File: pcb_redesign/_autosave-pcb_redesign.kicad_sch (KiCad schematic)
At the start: 6 parts, among them U1 ESP32-S3-WROOM-1

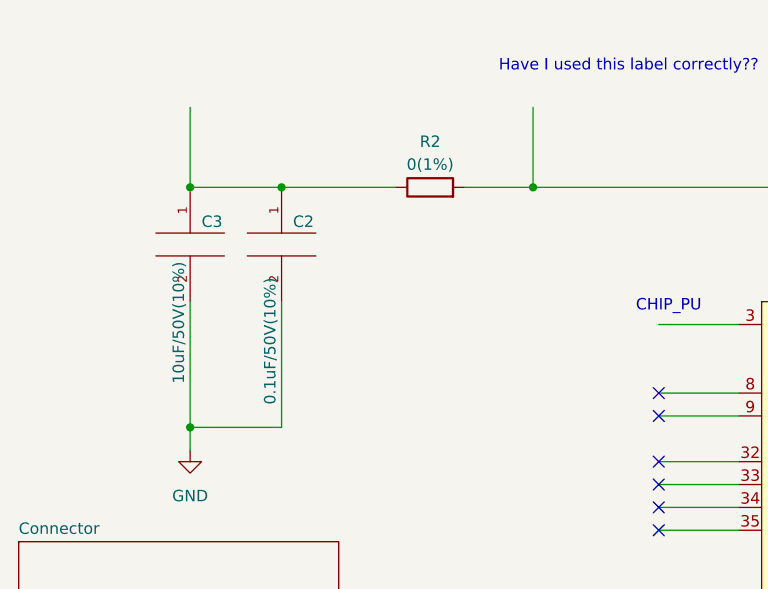
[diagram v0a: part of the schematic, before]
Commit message: 5.55pm 11.05
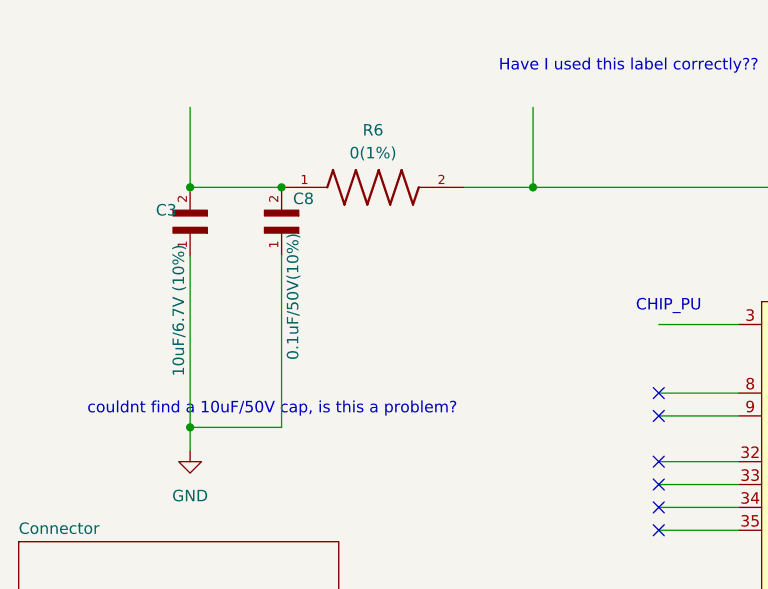
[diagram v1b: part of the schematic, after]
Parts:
- removed C2: 0.1uF/50V(10%), symbol pspice:C
- removed C3: 10uF/50V(10%), 10uF_cap_0805:CAPC2012X140N, symbol pspice:C
- removed R2: 0(1%), symbol Device:R
- added C3: 10uF/6.7V (10%), CAPC1608X90N, symbol 10uf_cap_0603:CL10A106MQ8NNNC
- added C8: 0.1uF/50V(10%), 1uF_cap_0603:CL10A105KB8NNNC, symbol 0.1uF_cap_0603:CL10B104KB8NNNL
- added R6: 0(1%), RESC1508X55N, symbol 0_ohm_0603:RMCF0603ZT0R00
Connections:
- net GND: now also C3.1, C8.1
- net at U1.2 (3V3): now also R6.2
- new net: C3.2, C8.2, R6.1
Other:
- note added: "couldnt find a 10uF/50V cap, is this a problem?"
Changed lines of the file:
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@@
 (kicad_sch (version 20230121) (generator eeschema)
   (paper "A4")
+  (junction (at 46.99 43.18) (diameter 0) (color 0 0 0 0)
+  )
   (junction (at 36.83 43.18) (diameter 0) (color 0 0 0 0)
   )
   (junction (at 36.83 69.85) (diameter 0) (color 0 0 0 0)
-  )
-  (junction (at 46.99 43.18) (diameter 0) (color 0 0 0 0)
   )
   (junction (at 66.04 175.26) (diameter 0) (color 0 0 0 0)
@@
     (stroke (width 0) (type default))
   )
+  (wire (pts (xy 88.9 129.54) (xy 97.79 129.54))
+    (stroke (width 0) (type default))
+  )
+  (wire (pts (xy 88.9 81.28) (xy 97.79 81.28))
+    (stroke (width 0) (type default))
+  )
+  (wire (pts (xy 88.9 68.58) (xy 97.79 68.58))
+    (stroke (width 0) (type default))
+  )
+  (wire (pts (xy 36.83 69.85) (xy 46.99 69.85))
+    (stroke (width 0) (type default))
+  )
+  (wire (pts (xy 189.23 129.54) (xy 199.39 129.54))
+    (stroke (width 0) (type default))
+  )
+  (wire (pts (xy 189.23 119.38) (xy 199.39 119.38))
+    (stroke (width 0) (type default))
+  )
   (wire (pts (xy 36.83 43.18) (xy 46.99 43.18))
     (stroke (width 0) (type default))
   )
-  (wire (pts (xy 88.9 129.54) (xy 97.79 129.54))
-    (stroke (width 0) (type default))
-  )
-  (wire (pts (xy 88.9 81.28) (xy 97.79 81.28))
-    (stroke (width 0) (type default))
-  )
-  (wire (pts (xy 88.9 68.58) (xy 97.79 68.58))
-    (stroke (width 0) (type default))
-  )
-  (wire (pts (xy 36.83 69.85) (xy 46.99 69.85))
-    (stroke (width 0) (type default))
-  )
-  (wire (pts (xy 189.23 129.54) (xy 199.39 129.54))
-    (stroke (width 0) (type default))
-  )
-  (wire (pts (xy 189.23 119.38) (xy 199.39 119.38))
-    (stroke (width 0) (type default))
-  )
   (wire (pts (xy 189.23 99.06) (xy 199.39 99.06))
     (stroke (width 0) (type default))
@@
     (stroke (width 0) (type default))
   )
-  (wire (pts (xy 46.99 43.18) (xy 59.69 43.18))
-    (stroke (width 0) (type default))
-  )
   (wire (pts (xy 36.83 69.85) (xy 36.83 72.39))
     (stroke (width 0) (type default))
@@
     (stroke (width 0) (type default))
   )
-  (wire (pts (xy 36.83 55.88) (xy 36.83 69.85))
+  (wire (pts (xy 36.83 50.8) (xy 36.83 69.85))
     (stroke (width 0) (type default))
   )
@@
     (stroke (width 0) (type default))
   )
-  (wire (pts (xy 46.99 55.88) (xy 46.99 69.85))
+  (wire (pts (xy 46.99 50.8) (xy 46.99 69.85))
     (stroke (width 0) (type default))
   )
@@
   )
   (text "Have I used this label correctly??" (at 71.12 30.48 0)
+    (effects (font (size 1.27 1.27)) (justify left bottom))
+  )
+  (text "couldnt find a 10uF/50V cap, is this a problem?" (at 25.4 68.58 0)
     (effects (font (size 1.27 1.27)) (justify left bottom))
   )
@@
     )
   )
-  (symbol (lib_id "pspice:C") (at 46.99 49.53 0) (unit 1)
+  (symbol (lib_id "10uf_cap_0603:CL10A106MQ8NNNC") (at 36.83 48.26 90) (unit 1)
     (in_bom yes) (on_board yes) (dnp no)
-    (property "Reference" "C2" (at 48.26 46.99 0)
-      (effects (font (size 1.27 1.27)) (justify left))
-    )
-    (property "Value" "0.1uF/50V(10%)" (at 45.72 67.31 90)
-      (effects (font (size 1.27 1.27)) (justify left))
-    )
-    (property "Footprint" "" (at 46.99 49.53 0)
-      (effects (font (size 1.27 1.27)) hide)
-    )
-    (property "Datasheet" "~" (at 46.99 49.53 0)
+    (property "Reference" "C3" (at 33.02 45.72 90)
+      (effects (font (size 1.27 1.27)) (justify right))
+    )
+    (property "Value" "10uF/6.7V (10%)" (at 35.56 49.53 0)
+      (effects (font (size 1.27 1.27)) (justify right))
+    )
+    (property "Footprint" "CAPC1608X90N" (at 36.83 48.26 0)
+      (effects (font (size 1.27 1.27)) (justify bottom) hide)
+    )
+    (property "Datasheet" "" (at 36.83 48.26 0)
       (effects (font (size 1.27 1.27)) hide)
     )
@@
       (project "pcb_redesign"
         (path "/fb030e39-7dd3-46a0-8379-c26b3ef1b0a0"
-          (reference "C2") (unit 1)
-        )
-      )
-    )
-  )
-  (symbol (lib_id "Device:R") (at 63.5 43.18 90) (unit 1)
-    (in_bom yes) (on_board yes) (dnp no) (fields_autoplaced)
-    (property "Reference" "R2" (at 63.5 38.1 90)
-      (effects (font (size 1.27 1.27)))
-    )
-    (property "Value" "0(1%)" (at 63.5 40.64 90)
-      (effects (font (size 1.27 1.27)))
-    )
-    (property "Footprint" "" (at 63.5 44.958 90)
-      (effects (font (size 1.27 1.27)) hide)
-    )
-    (property "Datasheet" "~" (at 63.5 43.18 0)
+          (reference "C3") (unit 1)
+        )
+      )
+    )
+  )
+  (symbol (lib_id "0.1uF_cap_0603:CL10B104KB8NNNL") (at 46.99 48.26 90) (unit 1)
+    (in_bom yes) (on_board yes) (dnp no)
+    (property "Reference" "C8" (at 48.26 44.45 90)
+      (effects (font (size 1.27 1.27)) (justify right))
+    )
+    (property "Value" "0.1uF/50V(10%)" (at 48.26 48.26 0)
+      (effects (font (size 1.27 1.27)) (justify right))
+    )
+    (property "Footprint" "1uF_cap_0603:CL10A105KB8NNNC" (at 46.99 48.26 0)
+      (effects (font (size 1.27 1.27)) (justify bottom) hide)
+    )
+    (property "Datasheet" "" (at 46.99 48.26 0)
       (effects (font (size 1.27 1.27)) hide)
     )
@@
       (project "pcb_redesign"
         (path "/fb030e39-7dd3-46a0-8379-c26b3ef1b0a0"
-          (reference "R2") (unit 1)
+          (reference "C8") (unit 1)
         )
       )
@@
         (path "/fb030e39-7dd3-46a0-8379-c26b3ef1b0a0"
           (reference "#PWR01") (unit 1)
-        )
-      )
-    )
-  )
-  (symbol (lib_id "pspice:C") (at 36.83 49.53 0) (unit 1)
-    (in_bom yes) (on_board yes) (dnp no)
-    (property "Reference" "C3" (at 38.1 46.99 0)
-      (effects (font (size 1.27 1.27)) (justify left))
-    )
-    (property "Value" "10uF/50V(10%)" (at 35.56 51.435 90)
-      (effects (font (size 1.27 1.27)) (justify right))
-    )
-    (property "Footprint" "10uF_cap_0805:CAPC2012X140N" (at 36.83 49.53 0)
-      (effects (font (size 1.27 1.27)) hide)
-    )
-    (property "Datasheet" "~" (at 36.83 49.53 0)
-      (effects (font (size 1.27 1.27)) hide)
-    )
-    (pin "1")
-    (pin "2")
-    (instances
-      (project "pcb_redesign"
-        (path "/fb030e39-7dd3-46a0-8379-c26b3ef1b0a0"
-          (reference "C3") (unit 1)
         )
       )
@@
         )
       )
+    )
+  )
+  (symbol (lib_id "0_ohm_0603:RMCF0603ZT0R00") (at 57.15 43.18 0) (unit 1)
+    (in_bom yes) (on_board yes) (dnp no) (fields_autoplaced)
+    (property "Reference" "R6" (at 57.15 36.83 0)
+      (effects (font (size 1.27 1.27)))
+    )
+    (property "Value" "0(1%)" (at 57.15 39.37 0)
+      (effects (font (size 1.27 1.27)))
+    )
+    (property "Footprint" "RESC1508X55N" (at 57.15 43.18 0)
+      (effects (font (size 1.27 1.27)) (justify bottom) hide)
+    )
+    (property "Datasheet" "" (at 57.15 43.18 0)
+      (effects (font (size 1.27 1.27)) hide)
+    )
+    (pin "1")
+    (pin "2")
+    (instances
+      (project "pcb_redesign"
+        (path "/fb030e39-7dd3-46a0-8379-c26b3ef1b0a0"
+          (reference "R6") (unit 1)
+        )
+      )
